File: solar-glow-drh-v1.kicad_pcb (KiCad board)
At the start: 4 copper layers, 50.8 x 88.9 mm, 37 parts, among them SW1 SW_F12340, SW2 slide OFF/ON/TINY

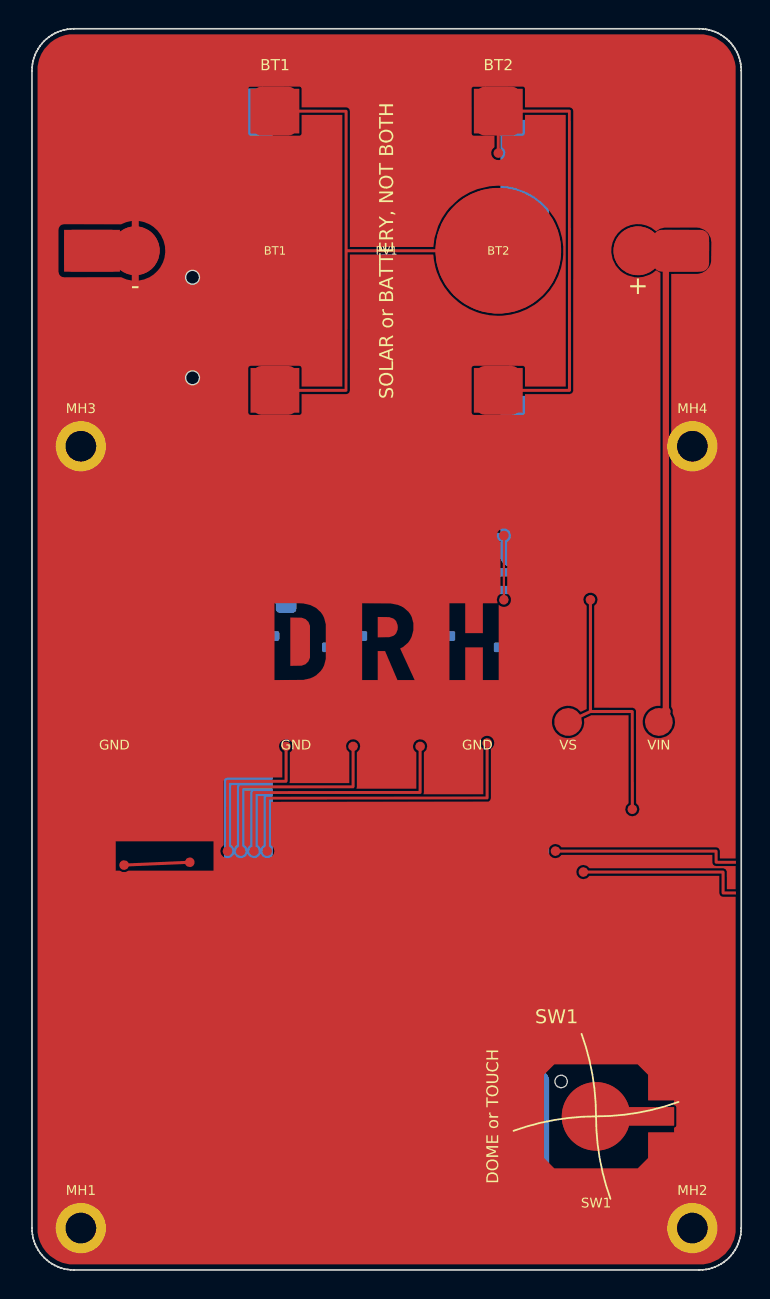
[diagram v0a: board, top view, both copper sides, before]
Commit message: Add files via upload
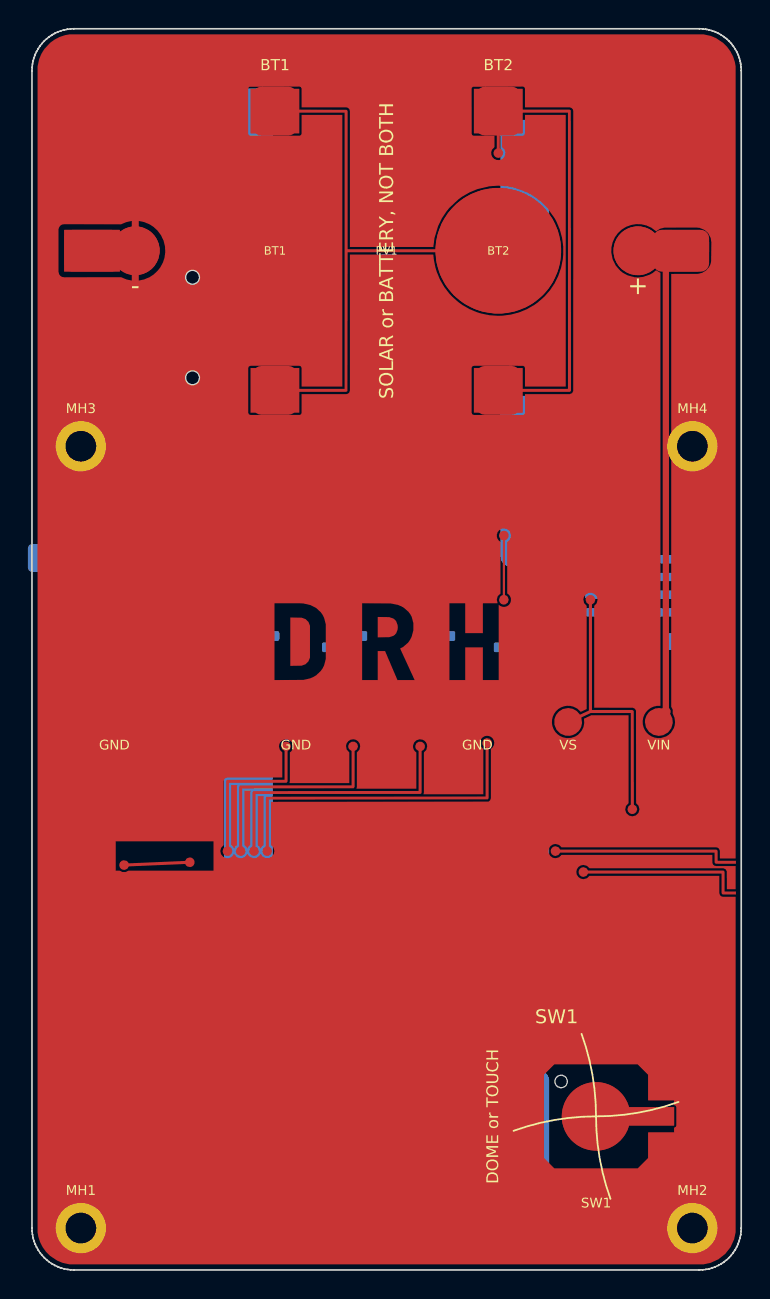
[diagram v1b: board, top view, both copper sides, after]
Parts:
- moved C3 50.5 mm to (12.0, 43.9)
- moved D1 48.9 mm to (44.0, 43.9)
- moved C2 47.4 mm to (8.00, 37.9)
- moved U2 12.1 mm to (43.0, 39.9)
- moved C1 10.9 mm to (5.00, 43.9)
- moved C4 9.14 mm to (47.5, 39.9)
- moved C5 7.91 mm to (7.00, 45.9)
- moved R5 7.91 mm to (3.00, 45.9)
- moved R6 7.91 mm to (5.00, 45.9)
- moved SJ1 6.02 mm to (13.0, 41.9)
- moved JP1 4.72 mm to (13.5, 37.9), turned to 90 degrees
- moved SW2 3.52 mm to (25.0, 84.9)
- moved U1 2.82 mm to (9.50, 40.9)
- moved J1 2.63 mm to (3.00, 37.9), turned to 90 degrees
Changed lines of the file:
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@@
   )
   (footprint "slide_OFF/ON/TINY" (layer "B.Cu")
-    (at 28.5 85.3)
+    (at 25.0 84.9 0)
     (attr smd)
     (fp_rect (start -3.3 -1.5) (end 3.3 1.5) (layer "B.CrtYd") (width 0.05) (fill none))
@@
   )
   (footprint "U1:QFN28" (layer "B.Cu")
-    (at 10.6 38.3 0)
+    (at 9.5 40.9 0)
     (attr smd)
     (fp_rect (start -2 -2) (end 2 2) (layer "B.CrtYd") (width 0.05) (fill none))
@@
   )
   (footprint "U2:SOIC8" (layer "B.Cu")
-    (at 31 38.3 0)
+    (at 43.0 39.9 0)
     (attr smd)
     (fp_rect (start -2.45 -1.95) (end 2.45 1.95) (layer "B.CrtYd") (width 0.05) (fill none))
@@
   )
   (footprint "D1:SOD" (layer "B.Cu")
-    (at 18 85.3 0)
+    (at 44.0 43.9 0)
     (attr smd)
     (fp_rect (start -1.85 -0.8) (end 1.85 0.8) (layer "B.CrtYd") (width 0.05) (fill none))
@@
   )
   (footprint "C1:0805" (layer "B.Cu")
-    (at 14.3 38.3 0)
+    (at 5.0 43.9 0)
     (attr smd)
     (fp_rect (start -1 -0.625) (end 1 0.625) (layer "B.CrtYd") (width 0.05) (fill none))
@@
   )
   (footprint "C2:0805" (layer "B.Cu")
-    (at 8 85.3 0)
+    (at 8.0 37.9 0)
     (attr smd)
     (fp_rect (start -1 -0.625) (end 1 0.625) (layer "B.CrtYd") (width 0.05) (fill none))
@@
   )
   (footprint "C3:0805" (layer "B.Cu")
-    (at 41 85.3 0)
+    (at 12.0 43.9 0)
     (attr smd)
     (fp_rect (start -1 -0.625) (end 1 0.625) (layer "B.CrtYd") (width 0.05) (fill none))
@@
   )
   (footprint "C4:0402" (layer "B.Cu")
-    (at 38.5 38.3 0)
+    (at 47.5 39.9 0)
     (attr smd)
     (fp_rect (start -0.5 -0.25) (end 0.5 0.25) (layer "B.CrtYd") (width 0.05) (fill none))
@@
   )
   (footprint "J1:PROG" (layer "B.Cu")
-    (at 5.6 38.3 0)
+    (at 3.0 37.9 90)
     (attr smd)
     (fp_text reference "J1" (at 0 0 0) (layer "B.SilkS")
@@
   )
   (footprint "JP1:PROG" (layer "B.Cu")
-    (at 18.2 38.3 0)
+    (at 13.5 37.9 90)
     (attr smd)
     (fp_text reference "JP1" (at 0 0 0) (layer "B.SilkS")
@@
   )
   (footprint "SJ1:0402" (layer "B.Cu")
-    (at 7.0 41.4 0)
+    (at 13.0 41.9 0)
     (attr smd)
     (fp_rect (start -0.5 -0.25) (end 0.5 0.25) (layer "B.CrtYd") (width 0.05) (fill none))
@@
   )
   (footprint "R5:0402" (layer "B.Cu")
-    (at 9.5 41.4 0)
+    (at 3.0 45.9 0)
     (attr smd)
     (fp_rect (start -0.5 -0.25) (end 0.5 0.25) (layer "B.CrtYd") (width 0.05) (fill none))
@@
   )
   (footprint "R6:0402" (layer "B.Cu")
-    (at 11.5 41.4 0)
+    (at 5.0 45.9 0)
     (attr smd)
     (fp_rect (start -0.5 -0.25) (end 0.5 0.25) (layer "B.CrtYd") (width 0.05) (fill none))
@@
   )
   (footprint "C5:0402" (layer "B.Cu")
-    (at 13.5 41.4 0)
-    (attr smd)
-    (fp_rect (start -0.5 -0.25) (end 0.5 0.25) (layer "B.CrtYd") (width 0.05) (fill none))
+    (at 7.0 45.9 0)
+    (attr smd)
+    (fp_rect (start -0.5 -0.25) (end 0.5 0.25) (layer "B.CrtYd") (width 0.05) (fill none))
